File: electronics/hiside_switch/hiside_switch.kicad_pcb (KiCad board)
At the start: 2 copper layers, 75 x 50 mm, 20 parts, among them J1 Screw_Terminal_01x02, J2 Screw_Terminal_01x02, J3 Conn_01x04_Pin, Q1 BC848, U2 BTS6163D

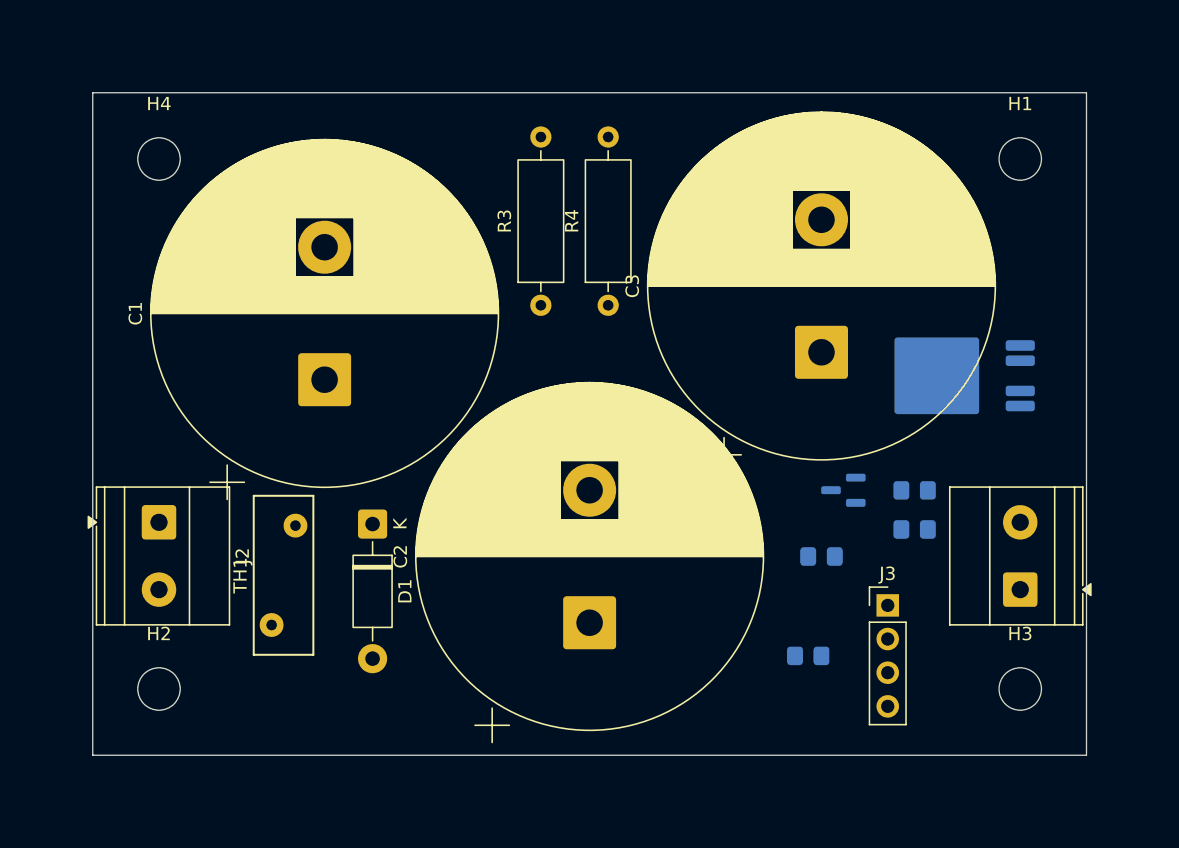
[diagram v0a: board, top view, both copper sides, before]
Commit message: routing completed
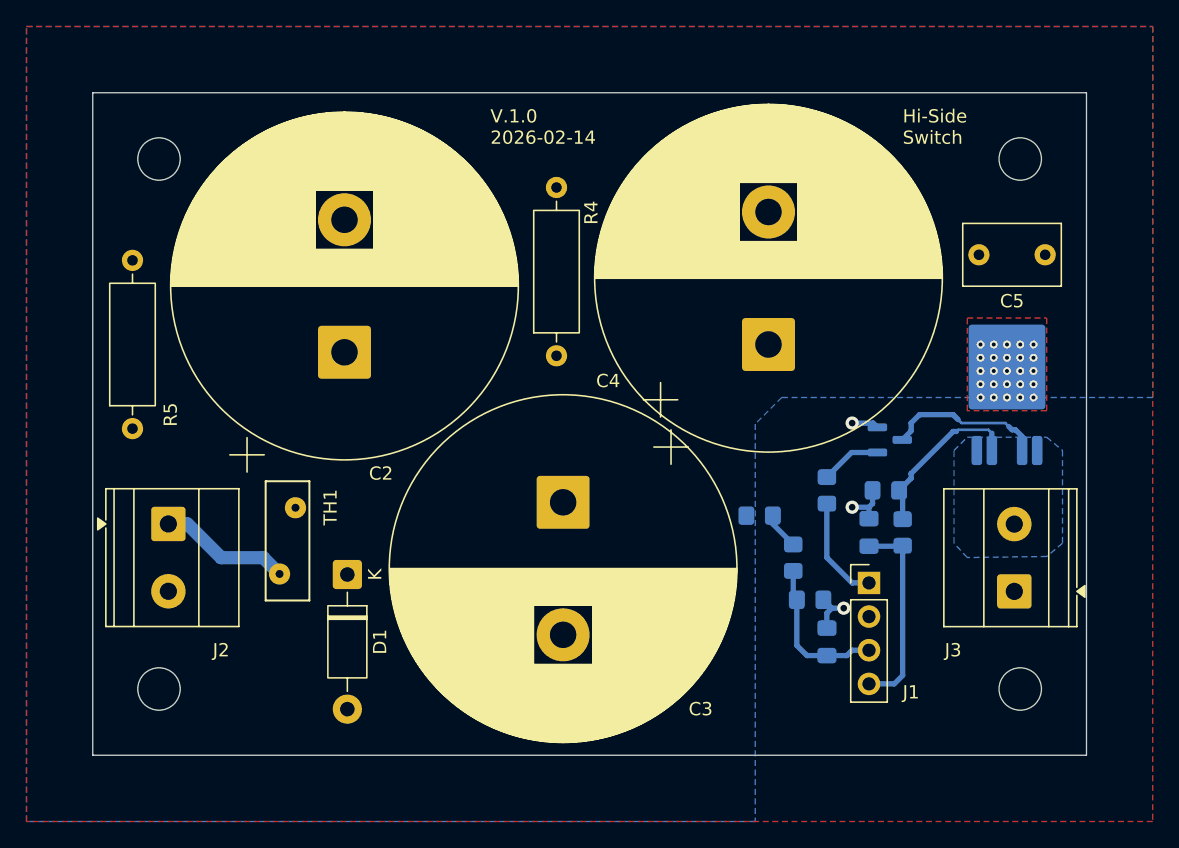
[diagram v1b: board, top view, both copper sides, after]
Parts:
- added C1: C, Capacitor_SMD:C_0805_2012Metric_Pad1.18x1.45mm_HandSolder, B.Cu at (105.4, 91.4)
- added C5: C, Capacitor_THT:C_Rect_L7.2mm_W4.5mm_P5.00mm_FKS2_FKP2_MKS2_MKP2, F.Cu at (121.9, 62.2)
- added C6: C, Capacitor_SMD:C_0805_2012Metric_Pad1.18x1.45mm_HandSolder, B.Cu at (108.6, 83.2)
- added R1: R, Resistor_SMD:R_0805_2012Metric_Pad1.20x1.40mm_HandSolder, B.Cu at (100.3, 81.9)
- added R7: R, Resistor_SMD:R_0805_2012Metric_Pad1.20x1.40mm_HandSolder, B.Cu at (111.1, 83.2)
- TH1: footprint Varistor:RV_Disc_D12mm_W4.5mm_P7.5mm -> Varistor:RV_Disc_D9mm_W3.3mm_P5mm
- moved R5 32.2 mm to (53.0, 75.3)
- moved R6 12.6 mm to (105.4, 80.0), turned to 90 degrees
- moved R3 11.4 mm to (104.1, 88.3)
- moved R2 9.40 mm to (102.9, 85.1), turned to 90 degrees
- moved C3 9.31 mm to (85.5, 80.9), turned to -90 degrees
- moved R8 6.96 mm to (109.9, 80.0)
- moved R4 5.45 mm to (85.0, 69.8)
- moved Q1 5.17 mm to (110.2, 76.2), turned to 0 degrees
- moved D1 4.26 mm to (69.2, 86.4)
- moved U1 4.08 mm to (119.0, 72.0), turned to 90 degrees
- moved C4 4.04 mm to (101.0, 69.0)
- moved C2 2.56 mm to (69.0, 69.6)
- moved J1 2.21 mm to (108.6, 87.0)
- moved TH1 1.35 mm to (65.3, 81.3)
- moved J2 0.72 mm to (55.7, 82.5)
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- renumbered C1 to C2, C2 to C3, C3 to C4, J3 to J1, J1 to J3, R6 to R2, R5 to R3, R3 to R5, R2 to R6, R1 to R8, U2 to U1
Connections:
- net Net-(J1-Pin_2) renamed /pout
- C2 pad 1: Net-(D1-K) -> VCC
- C2 pad 2: Net-(D1-A) -> GND
- C3 pad 1: Net-(D1-K) -> VCC
- C3 pad 2: Net-(D1-A) -> GND
- C4 pad 1: Net-(D1-K) -> VCC
- C4 pad 2: Net-(D1-A) -> GND
- D1 pad 1: Net-(D1-K) -> VCC
- D1 pad 2: Net-(D1-A) -> GND
- J1 pad 1: Net-(J3-Pin_1) -> Net-(J1-Pin_1)
- J1 pad 2: Net-(J3-Pin_2) -> GND
- J1 pad 3: Net-(J3-Pin_3) -> Net-(J1-Pin_3)
- J1 pad 4: Net-(D1-A) -> Net-(J1-Pin_4)
- J2 pad 2: Net-(D1-A) -> GND
- J3 pad 1: Net-(D1-A) -> GND
- Q1 pad 2: Net-(D1-A) -> GND
- R2 pad 1: Net-(J3-Pin_1) -> Net-(J1-Pin_3)
- R2 pad 2: Net-(D1-K) -> Net-(R1-Pad1)
- R3 pad 1: Net-(D1-A) -> GND
- R3 pad 2: Net-(J3-Pin_1) -> Net-(J1-Pin_3)
- R4 pad 1: Net-(D1-K) -> VCC
- R4 pad 2: Net-(D1-A) -> GND
- R5 pad 1: Net-(D1-K) -> VCC
- R5 pad 2: Net-(D1-A) -> GND
- R6 pad 1: Net-(J3-Pin_2) -> Net-(J1-Pin_1)
- R8 pad 1: Net-(J3-Pin_3) -> Net-(U1-IS)
- R8 pad 2: Net-(D1-A) -> GND
- TH1 pad 1: Net-(D1-K) -> VCC
- U1 pad 3: Net-(D1-K) -> VCC
- U1 pad 4: Net-(J3-Pin_3) -> Net-(U1-IS)
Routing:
- net Net-(J1-Pin_4): track 0.00 -> 15.2 mm
- net Net-(Q1-C): track 0.00 -> 12.9 mm
- net Net-(U1-IS): track 0.00 -> 12.8 mm
- net Net-(J1-Pin_3): track 0.00 -> 11.7 mm
- net Net-(J2-Pin_1): track 0.00 -> 9.96 mm
- net GND: track 0.00 -> 9.01 mm, vias 0 -> 3
- net Net-(J1-Pin_1): track 0.00 -> 8.04 mm
- net Net-(Q1-B): track 0.00 -> 4.58 mm
- net Net-(R1-Pad1): track 0.00 -> 2.81 mm
- net VCC: vias 0 -> 25
- added copper zone on B.Cu, net /pout
- added copper zone on F.Cu, net GND
- added copper zone on B.Cu, net VCC
- added copper zone on F.Cu, net VCC
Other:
- board text added: "Hi-Side Switch"
- board text added: "V.1.0 2026-02-14"
